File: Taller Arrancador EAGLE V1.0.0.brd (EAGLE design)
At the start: 17.3 x 13.3 mm, 14 parts, among them IC1 VS1838BB, U2 ATTINY412-SSNR

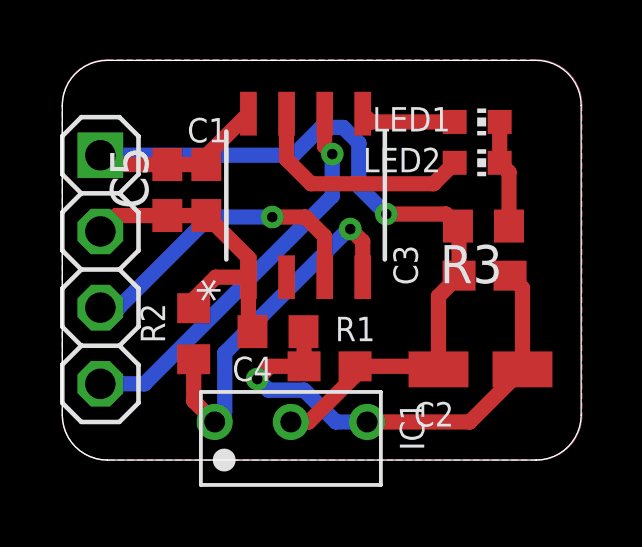
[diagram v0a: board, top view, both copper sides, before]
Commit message: Add files via upload
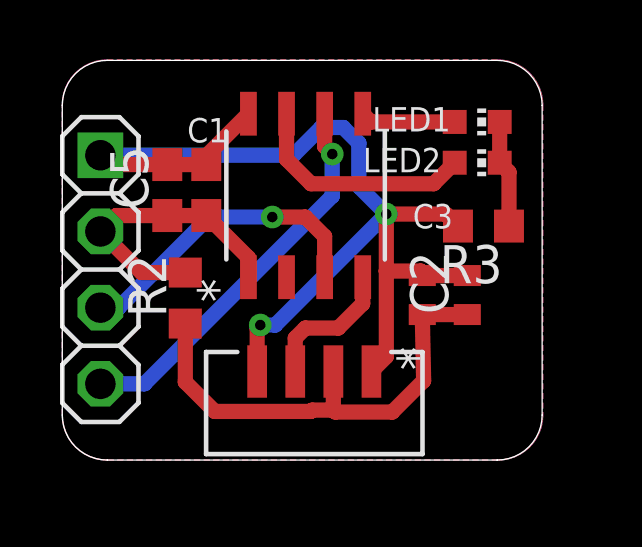
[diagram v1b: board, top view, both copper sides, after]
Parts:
- removed C4: 10uF, rcl:C0603
- removed IC1: VS1838BB, LFN-VS1838B_Infrared_Sensor:VS1838B
- removed R1: 100E, rcl:R0603
- added U1: TSOP75338WTT, receptorir38:TSOP75338WTT_VIS
- C2: value 100uF -> 0.1uF; device rcl:CT3216 -> rcl:C0402
- C3: device rcl:C0603 -> rcl:C0402
- R2: value 22K -> 100
- moved C2 2.52 mm to (13.5, 5.50), turned to 90 degrees
- moved C3 2.17 mm to (12.0, 5.50), turned to 90 degrees
- moved GOLD_ORB_SM1 1.77 mm to (12.3, 4.90)
- moved R2 1.22 mm to (4.10, 5.40)
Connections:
- removed net N$1: C2.+, C3.1, C4.1, IC1.VCC, R1.1
- new net N$2: C2.1, C3.1, R2.1, U1.2
- net +5V: no longer R1.2
- net GND: now also C2.2, U1.1, U1.4; no longer C2.-, C4.2, IC1.GND
- net OUT: now also U1.3; no longer IC1.OUT, R2.1
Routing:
- net N$1: track 16.5 -> 0.00 mm, vias 1 -> 0
- net N$2: track 0.00 -> 15.8 mm
- net OUT: track 12.5 -> 4.72 mm, vias 1 -> 0
- net GND: track 31.4 -> 36.1 mm, vias 1 -> 2
- net +5V: track 10.9 -> 9.78 mm
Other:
- board size 17.3 x 13.3 mm -> 16 x 13.3 mm
- board text added: "C:/Users/SYSTEMS/Downloads/logo.bmp"
- board text added: "Diseñado en Méixco por Sol"
- board text added: "y Nomada-e"
- board text removed: "Diseñado en México por Sol y Nomada-e"
